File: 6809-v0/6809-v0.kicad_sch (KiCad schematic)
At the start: 7 parts, among them U1 MC68B09, U2 2764, U3 W65C51NxP, U4 W65C22NxP, U5 CY62256-70PC, U6 CY62256-70PC, Y1 8MHz Xtal

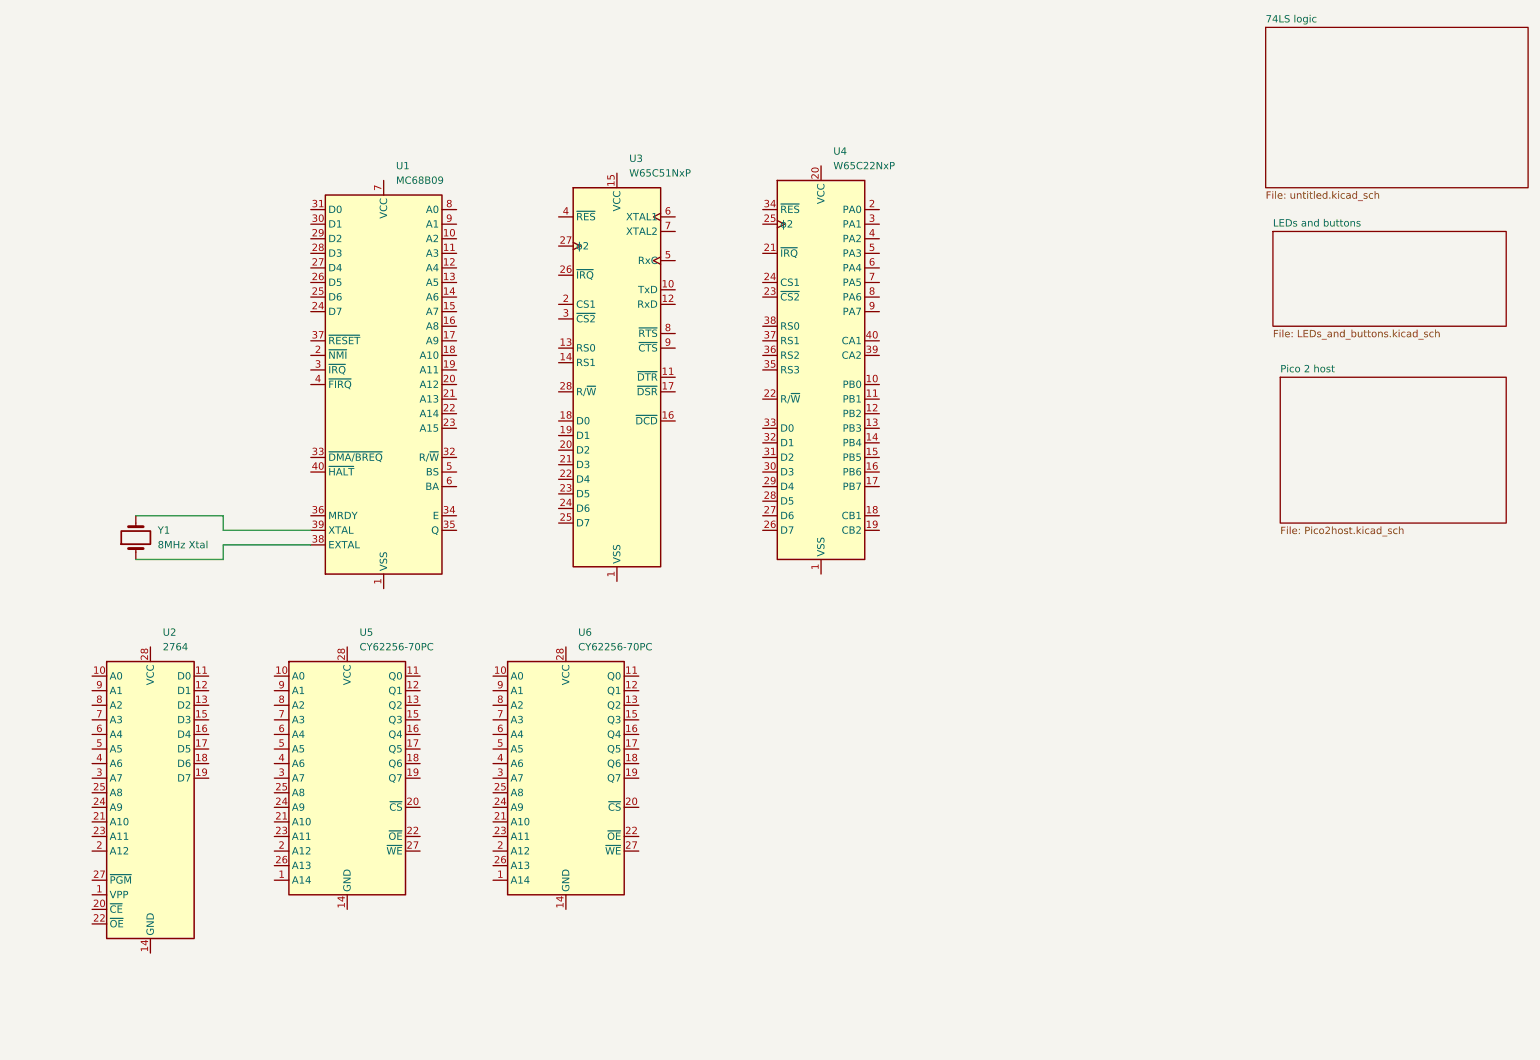
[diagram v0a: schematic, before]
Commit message: First checking of 6809 board:
- KiCad 9.0.5
- prior to upgrade
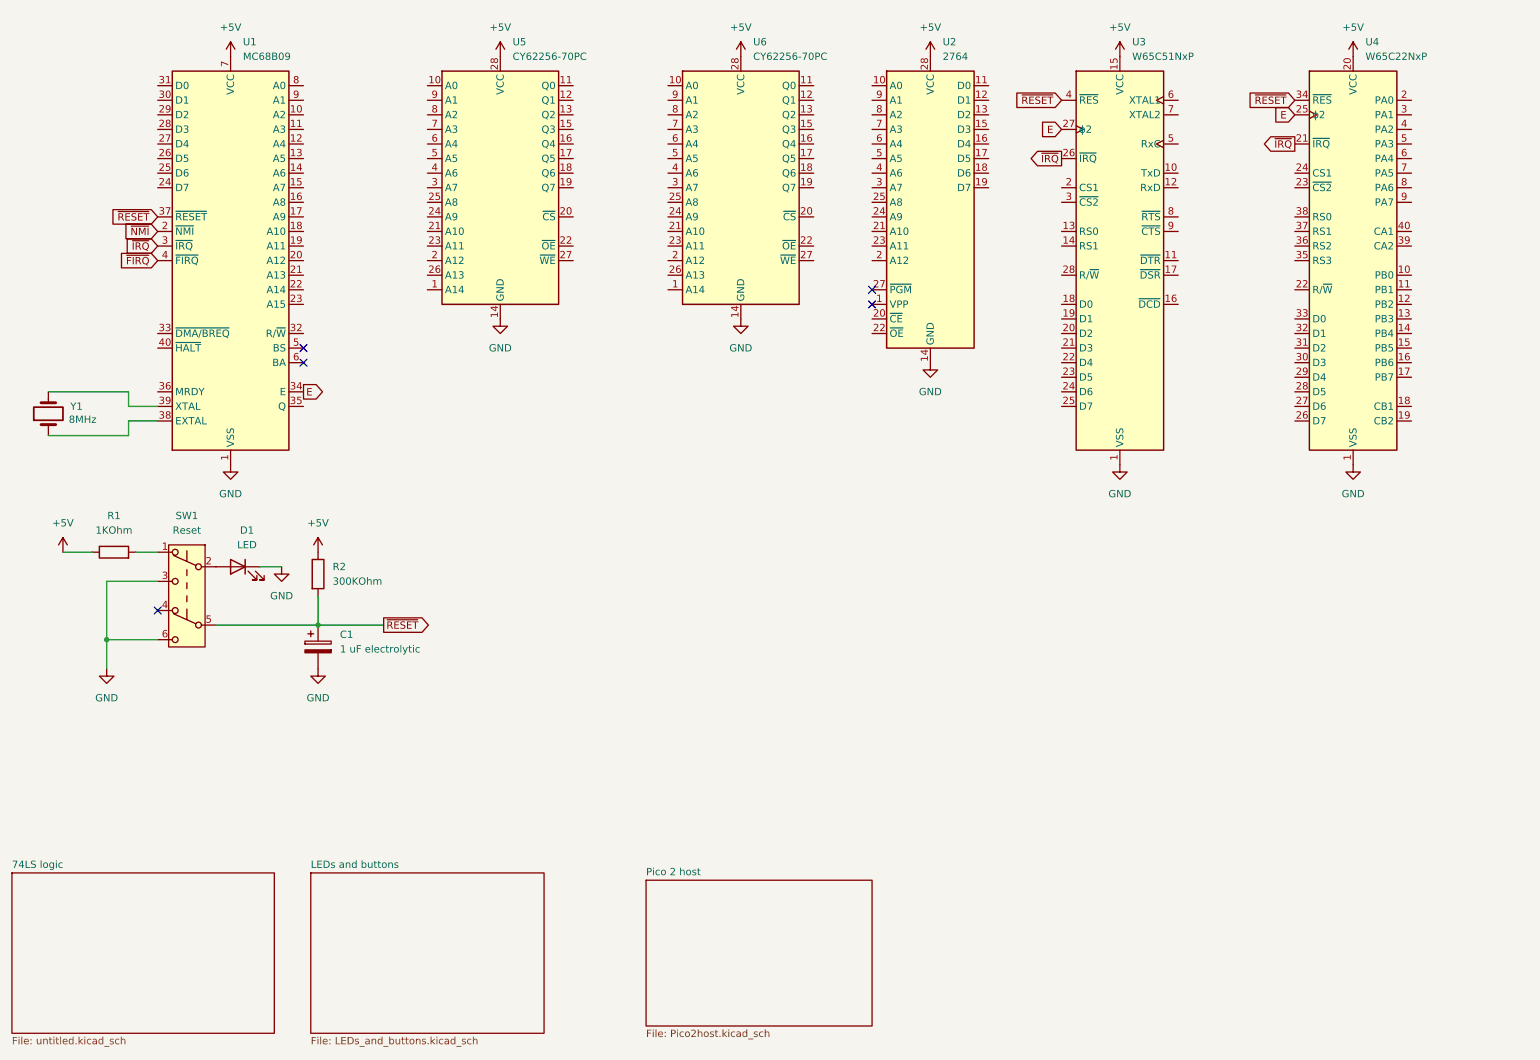
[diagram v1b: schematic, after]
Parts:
- added C1: 1 uF electrolytic, symbol Device:C_Polarized
- added D1: LED, symbol Device:LED
- added R1: 1KOhm, symbol Device:R
- added R2: 300KOhm, symbol Device:R
- added SW1: Reset, symbol Switch:SW_Push_DPDT
- Y1: value 8MHz Xtal -> 8MHz
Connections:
- net GND: now reaches U3.1 (VSS)
- net GND: now also U1.1 (VSS), U2.14 (GND), U4.1 (VSS), U5.14 (GND), U6.14 (GND), C1.2, D1.1 (K), SW1.3 (C), SW1.6 (C)
- net +5V: now reaches U3.15 (VCC)
- net +5V: now also U1.7 (VCC), U2.28 (VCC), U4.20 (VCC), U5.28 (VCC), U6.28 (VCC), R1.1, R2.1
- net ~{IRQ}: now reaches U3.26 (~{IRQ})
- net ~{IRQ}: now also U1.3 (~{IRQ}), U4.21 (~{IRQ})
- net E: now reaches U3.27 (ϕ2)
- net E: now also U1.34 (E), U4.25 (ϕ2)
- net ~{RESET}: now reaches U3.4 (~{RES})
- net ~{RESET}: now also U1.37 (~{RESET}), U4.34 (~{RES}), C1.1, R2.2, SW1.5 (B)
- net ~{NMI}: now reaches U1.2 (~{NMI})
- net ~{FIRQ}: now reaches U1.4 (~{FIRQ})
- new net: R1.2, SW1.1 (A)
- new net: D1.2 (A), SW1.2 (B)
- no-connect marks 0 -> 5
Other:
- moved on the sheet: U1, U2, U3, U4, U5, U6, Y1
